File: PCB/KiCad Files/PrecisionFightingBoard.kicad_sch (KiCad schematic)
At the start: 14 parts, among them J1 Conn_01x04_Male, J10 ST01x05, J3 Conn_01x14_Socket, J4 Conn_01x14_Socket, J5 Screw_Terminal_01x03, J6 Conn_02x10_Odd_Even, J7 ST01x05, J8 ST01x05, J9 ST01x05, U1 Teensy4.0

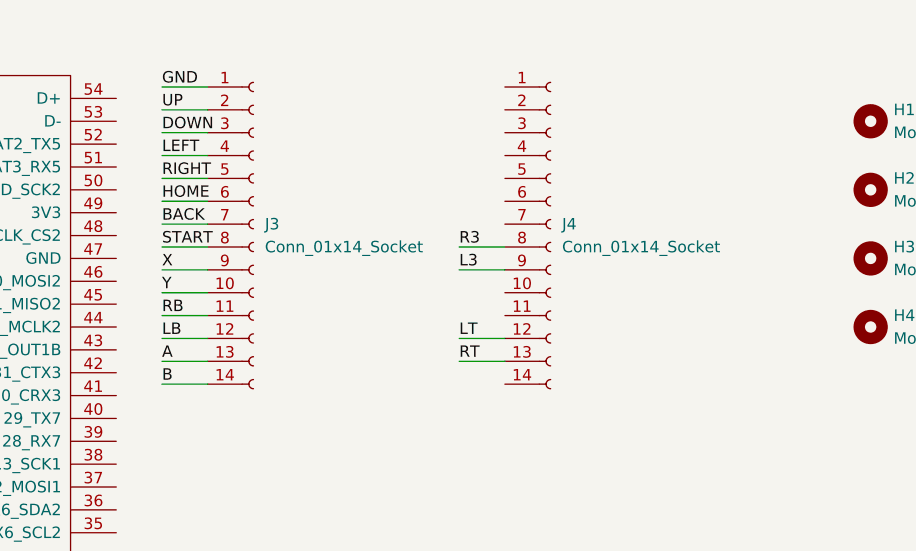
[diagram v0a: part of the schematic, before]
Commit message: fix pcb
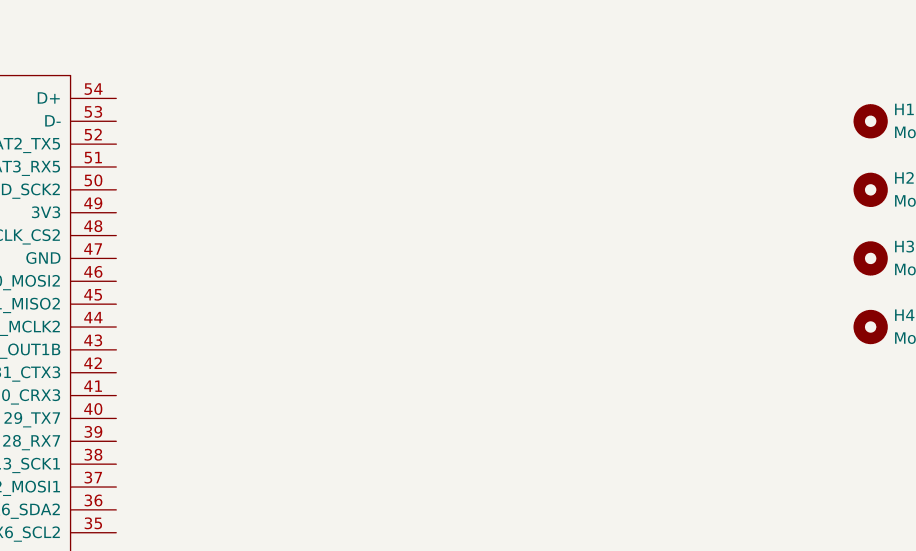
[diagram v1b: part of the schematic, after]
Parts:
- removed J3, J4: Conn_01x14_Socket, Connector_PinSocket_2.54mm:PinSocket_1x14_P2.54mm_Vertical, symbol Connector:Conn_01x14_Socket
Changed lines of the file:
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@@
-    (stroke (width 0) (type default))
-  )
-  (wire (pts (xy 180.34 41.91) (xy 185.42 41.91))
     (stroke (width 0) (type default))
   )
@@
     (stroke (width 0) (type default))
   )
-  (wire (pts (xy 180.34 26.67) (xy 185.42 26.67))
-    (stroke (width 0) (type default))
-  )
-  (wire (pts (xy 180.34 46.99) (xy 185.42 46.99))
-    (stroke (width 0) (type default))
-  )
   (wire (pts (xy 114.3 25.4) (xy 119.38 25.4))
     (stroke (width 0) (type default))
@@
     (stroke (width 0) (type default))
   )
-  (wire (pts (xy 180.34 36.83) (xy 185.42 36.83))
-    (stroke (width 0) (type default))
-  )
   (wire (pts (xy 92.71 55.88) (xy 85.09 55.88))
     (stroke (width 0) (type default))
@@
     (stroke (width 0) (type default))
   )
-  (wire (pts (xy 213.36 52.07) (xy 218.44 52.07))
-    (stroke (width 0) (type default))
-  )
   (wire (pts (xy 92.71 48.26) (xy 85.09 48.26))
     (stroke (width 0) (type default))
@@
     (stroke (width 0) (type default))
   )
-  (wire (pts (xy 180.34 24.13) (xy 185.42 24.13))
-    (stroke (width 0) (type default))
-  )
   (wire (pts (xy 114.3 22.86) (xy 119.38 22.86))
     (stroke (width 0) (type default))
@@
     (stroke (width 0) (type default))
   )
-  (wire (pts (xy 180.34 39.37) (xy 185.42 39.37))
-    (stroke (width 0) (type default))
-  )
   (wire (pts (xy 63.5 55.88) (xy 72.39 55.88))
     (stroke (width 0) (type default))
@@
     (stroke (width 0) (type default))
   )
-  (wire (pts (xy 180.34 29.21) (xy 185.42 29.21))
-    (stroke (width 0) (type default))
-  )
-  (wire (pts (xy 180.34 44.45) (xy 185.42 44.45))
-    (stroke (width 0) (type default))
-  )
   (wire (pts (xy 35.56 26.67) (xy 30.48 26.67))
     (stroke (width 0) (type default))
   )
-  (wire (pts (xy 180.34 52.07) (xy 185.42 52.07))
-    (stroke (width 0) (type default))
-  )
-  (wire (pts (xy 180.34 54.61) (xy 185.42 54.61))
-    (stroke (width 0) (type default))
-  )
   (wire (pts (xy 114.3 40.64) (xy 119.38 40.64))
     (stroke (width 0) (type default))
@@
     (stroke (width 0) (type default))
   )
-  (wire (pts (xy 213.36 49.53) (xy 218.44 49.53))
-    (stroke (width 0) (type default))
-  )
   (wire (pts (xy 35.56 39.37) (xy 30.48 39.37))
     (stroke (width 0) (type default))
@@
     (stroke (width 0) (type default))
   )
-  (wire (pts (xy 180.34 34.29) (xy 185.42 34.29))
-    (stroke (width 0) (type default))
-  )
   (wire (pts (xy 63.5 48.26) (xy 72.39 48.26))
     (stroke (width 0) (type default))
@@
     (stroke (width 0) (type default))
   )
-  (wire (pts (xy 180.34 31.75) (xy 185.42 31.75))
-    (stroke (width 0) (type default))
-  )
   (wire (pts (xy 92.71 58.42) (xy 85.09 58.42))
     (stroke (width 0) (type default))
@@
     (stroke (width 0) (type default))
   )
-  (wire (pts (xy 180.34 49.53) (xy 185.42 49.53))
-    (stroke (width 0) (type default))
-  )
   (wire (pts (xy 92.71 43.18) (xy 85.09 43.18))
     (stroke (width 0) (type default))
@@
     (stroke (width 0) (type default))
   )
-  (wire (pts (xy 213.36 39.37) (xy 218.44 39.37))
-    (stroke (width 0) (type default))
-  )
   (wire (pts (xy 35.56 59.69) (xy 30.48 59.69))
     (stroke (width 0) (type default))
@@
     (stroke (width 0) (type default))
   )
-  (wire (pts (xy 180.34 21.59) (xy 185.42 21.59))
-    (stroke (width 0) (type default))
-  )
   (wire (pts (xy 114.3 35.56) (xy 119.38 35.56))
     (stroke (width 0) (type default))
@@
     (stroke (width 0) (type default))
   )
-  (wire (pts (xy 213.36 41.91) (xy 218.44 41.91))
-    (stroke (width 0) (type default))
-  )
   (wire (pts (xy 35.56 62.23) (xy 30.48 62.23))
     (stroke (width 0) (type default))
@@
     (effects (font (size 1.27 1.27)) (justify left bottom))
   )
-  (label "X" (at 180.34 41.91 0) (fields_autoplaced)
-    (effects (font (size 1.27 1.27)) (justify left bottom))
-  )
   (label "GND" (at 31.115 36.83 0) (fields_autoplaced)
     (effects (font (size 1.27 1.27)) (justify left bottom))
@@
     (effects (font (size 1.27 1.27)) (justify left bottom))
   )
-  (label "BACK" (at 180.34 36.83 0) (fields_autoplaced)
-    (effects (font (size 1.27 1.27)) (justify left bottom))
-  )
   (label "LEFT" (at 114.3 30.48 0) (fields_autoplaced)
     (effects (font (size 1.27 1.27)) (justify left bottom))
@@
     (effects (font (size 1.27 1.27)) (justify left bottom))
   )
-  (label "RB" (at 180.34 46.99 0) (fields_autoplaced)
-    (effects (font (size 1.27 1.27)) (justify left bottom))
-  )
   (label "R3" (at 55.88 102.87 0) (fields_autoplaced)
     (effects (font (size 1.27 1.27)) (justify left bottom))
   )
-  (label "DOWN" (at 180.34 26.67 0) (fields_autoplaced)
-    (effects (font (size 1.27 1.27)) (justify left bottom))
-  )
   (label "GND" (at 85.725 38.1 0) (fields_autoplaced)
     (effects (font (size 1.27 1.27)) (justify left bottom))
@@
     (effects (font (size 1.27 1.27)) (justify left bottom))
   )
-  (label "RT" (at 213.36 52.07 0) (fields_autoplaced)
-    (effects (font (size 1.27 1.27)) (justify left bottom))
-  )
-  (label "GND" (at 180.34 21.59 0) (fields_autoplaced)
-    (effects (font (size 1.27 1.27)) (justify left bottom))
-  )
-  (label "START" (at 180.34 39.37 0) (fields_autoplaced)
-    (effects (font (size 1.27 1.27)) (justify left bottom))
-  )
-  (label "HOME" (at 180.34 34.29 0) (fields_autoplaced)
-    (effects (font (size 1.27 1.27)) (justify left bottom))
-  )
   (label "LT" (at 114.3 76.2 0) (fields_autoplaced)
     (effects (font (size 1.27 1.27)) (justify left bottom))
   )
-  (label "R3" (at 213.36 39.37 0) (fields_autoplaced)
-    (effects (font (size 1.27 1.27)) (justify left bottom))
-  )
-  (label "L3" (at 213.36 41.91 0) (fields_autoplaced)
-    (effects (font (size 1.27 1.27)) (justify left bottom))
-  )
-  (label "RIGHT" (at 180.34 31.75 0) (fields_autoplaced)
-    (effects (font (size 1.27 1.27)) (justify left bottom))
-  )
   (label "RB" (at 69.215 48.26 0) (fields_autoplaced)
     (effects (font (size 1.27 1.27)) (justify left bottom))
   )
-  (label "Y" (at 180.34 44.45 0) (fields_autoplaced)
-    (effects (font (size 1.27 1.27)) (justify left bottom))
-  )
   (label "BACK" (at 85.725 53.34 0) (fields_autoplaced)
     (effects (font (size 1.27 1.27)) (justify left bottom))
@@
     (effects (font (size 1.27 1.27)) (justify left bottom))
   )
-  (label "LEFT" (at 180.34 29.21 0) (fields_autoplaced)
-    (effects (font (size 1.27 1.27)) (justify left bottom))
-  )
   (label "L3" (at 34.925 101.6 0) (fields_autoplaced)
     (effects (font (size 1.27 1.27)) (justify left bottom))
@@
     (effects (font (size 1.27 1.27)) (justify left bottom))
   )
-  (label "LT" (at 213.36 49.53 0) (fields_autoplaced)
-    (effects (font (size 1.27 1.27)) (justify left bottom))
-  )
   (label "LB" (at 31.115 54.61 0) (fields_autoplaced)
     (effects (font (size 1.27 1.27)) (justify left bottom))
@@
     (effects (font (size 1.27 1.27)) (justify left bottom))
   )
-  (label "LB" (at 180.34 49.53 0) (fields_autoplaced)
-    (effects (font (size 1.27 1.27)) (justify left bottom))
-  )
   (label "RIGHT" (at 31.115 31.75 0) (fields_autoplaced)
     (effects (font (size 1.27 1.27)) (justify left bottom))
   )
-  (label "A" (at 180.34 52.07 0) (fields_autoplaced)
-    (effects (font (size 1.27 1.27)) (justify left bottom))
-  )
   (label "GND" (at 34.925 106.68 0) (fields_autoplaced)
     (effects (font (size 1.27 1.27)) (justify left bottom))
@@
     (effects (font (size 1.27 1.27)) (justify left bottom))
   )
-  (label "UP" (at 180.34 24.13 0) (fields_autoplaced)
-    (effects (font (size 1.27 1.27)) (justify left bottom))
-  )
   (label "LT" (at 31.115 67.31 0) (fields_autoplaced)
     (effects (font (size 1.27 1.27)) (justify left bottom))
@@
   )
   (label "DOWN" (at 114.3 27.94 0) (fields_autoplaced)
-    (effects (font (size 1.27 1.27)) (justify left bottom))
-  )
-  (label "B" (at 180.34 54.61 0) (fields_autoplaced)
     (effects (font (size 1.27 1.27)) (justify left bottom))
   )
@@
         )
       )
-    )
-  )
-  (symbol (lib_id "Connector:Conn_01x14_Socket") (at 190.5 36.83 0) (unit 1)
-    (in_bom yes) (on_board yes) (dnp no) (fields_autoplaced)
-    (property "Reference" "J3" (at 191.77 36.83 0)
-      (effects (font (size 1.27 1.27)) (justify left))
-    )
-    (property "Value" "Conn_01x14_Socket" (at 191.77 39.37 0)
-      (effects (font (size 1.27 1.27)) (justify left))
-    )
-    (property "Footprint" "Connector_PinSocket_2.54mm:PinSocket_1x14_P2.54mm_Vertical" (at 190.5 36.83 0)
-      (effects (font (size 1.27 1.27)) hide)
-    )
-    (property "Datasheet" "~" (at 190.5 36.83 0)
-      (effects (font (size 1.27 1.27)) hide)
-    )
-    (pin "1")
-    (pin "10")
-    (pin "11")
-    (pin "12")
-    (pin "13")
-    (pin "14")
-    (pin "2")
-    (pin "3")
-    (pin "4")
-    (pin "5")
-    (pin "6")
-    (pin "7")
-    (pin "8")
-    (pin "9")
-    (instances
-      (project "PrecisionFightingBoard"
-        (path "/01d790aa-01e7-46c4-a23c-7deb91137dd0"
-          (reference "J3") (unit 1)
-        )
-      )
-    )
-  )
-  (symbol (lib_id "Connector:Conn_01x14_Socket") (at 223.52 36.83 0) (unit 1)
-    (in_bom yes) (on_board yes) (dnp no) (fields_autoplaced)
-    (property "Reference" "J4" (at 224.79 36.83 0)
-      (effects (font (size 1.27 1.27)) (justify left))
-    )
-    (property "Value" "Conn_01x14_Socket" (at 224.79 39.37 0)
-      (effects (font (size 1.27 1.27)) (justify left))
-    )
-    (property "Footprint" "Connector_PinSocket_2.54mm:PinSocket_1x14_P2.54mm_Vertical" (at 223.52 36.83 0)
-      (effects (font (size 1.27 1.27)) hide)
-    )
-    (property "Datasheet" "~" (at 223.52 36.83 0)
-      (effects (font (size 1.27 1.27)) hide)
-    )
-    (pin "1")
-    (pin "10")
-    (pin "11")
-    (pin "12")
-    (pin "13")
-    (pin "14")
-    (pin "2")
-    (pin "3")
-    (pin "4")
-    (pin "5")
-    (pin "6")
-    (pin "7")
-    (pin "8")
-    (pin "9")
-    (instances
-      (project "PrecisionFightingBoard"
-        (path "/01d790aa-01e7-46c4-a23c-7deb91137dd0"
-          (reference "J4") (unit 1)
-        )
-      )
